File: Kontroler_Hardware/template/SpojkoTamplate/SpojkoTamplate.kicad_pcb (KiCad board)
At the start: 2 copper layers, 139.7 x 63.5 mm, 1 part, among them J1 CONN_01X40

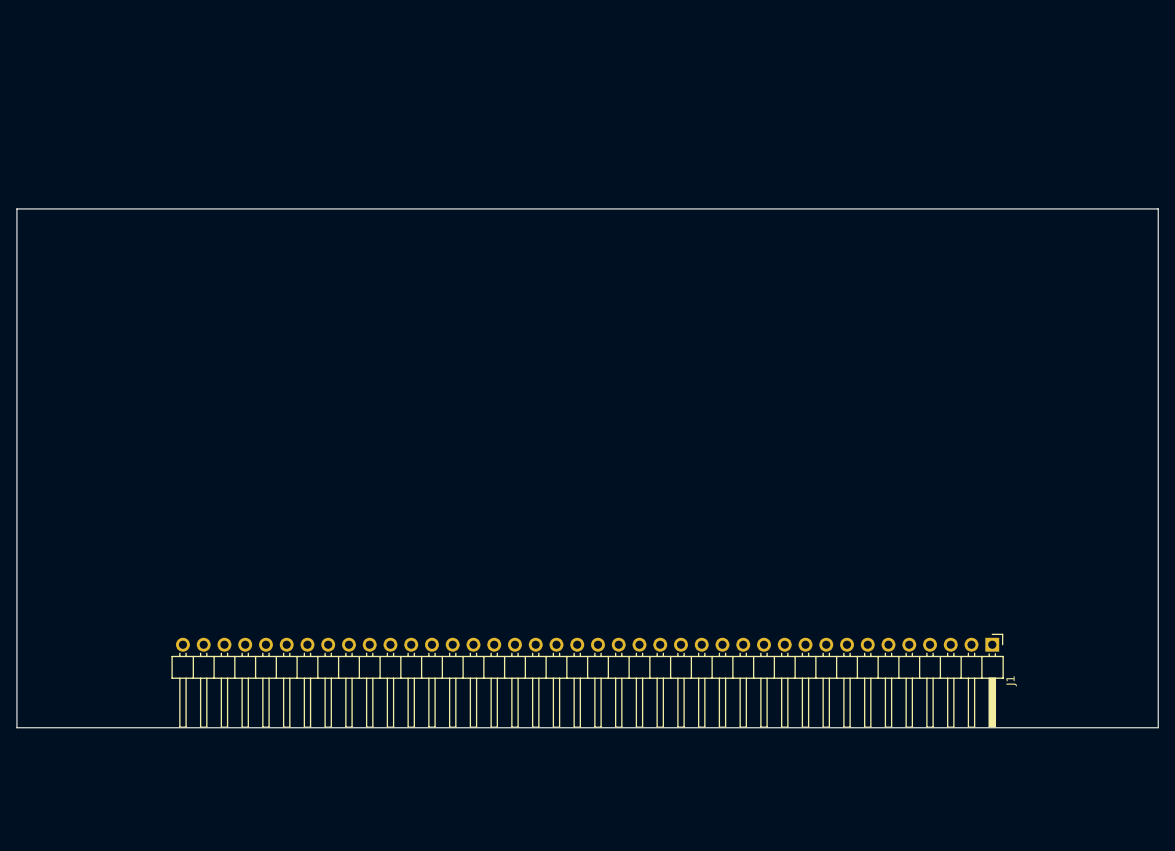
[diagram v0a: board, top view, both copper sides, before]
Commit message: Finish templates
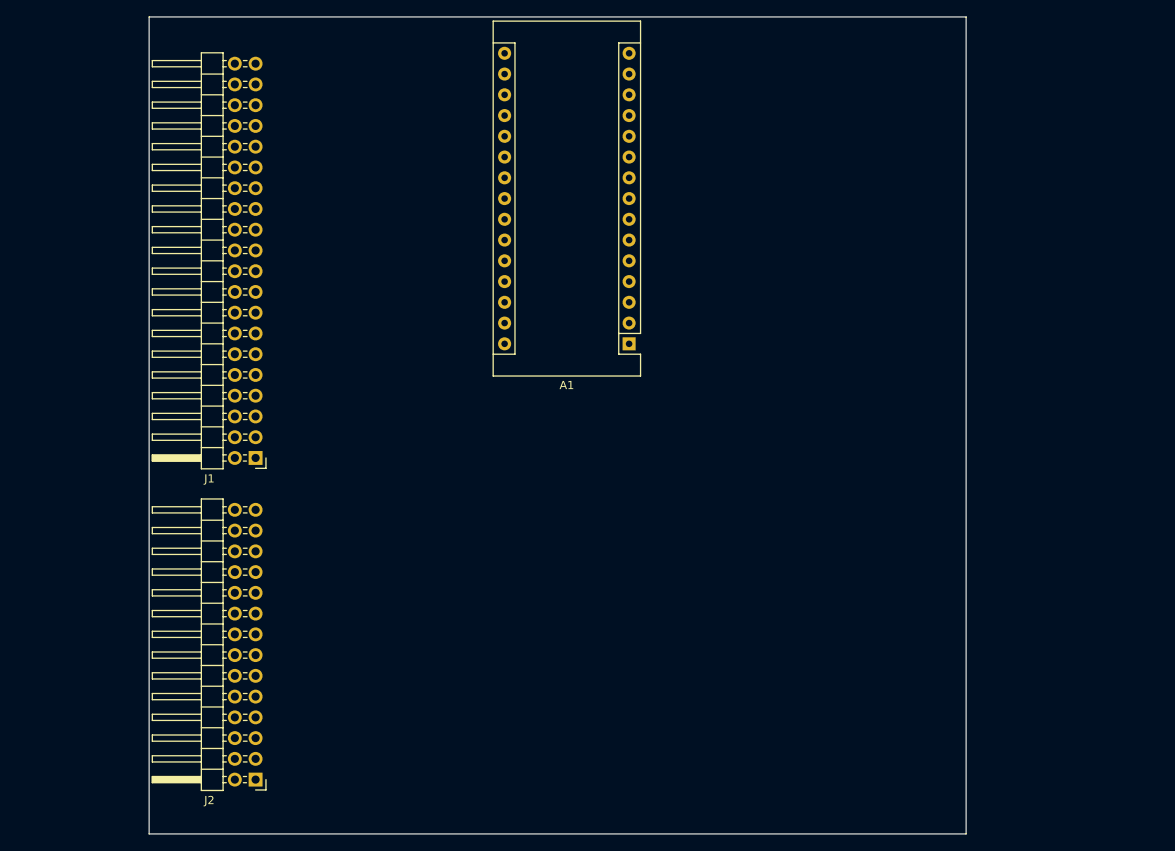
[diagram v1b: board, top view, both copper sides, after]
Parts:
- added A1: Arduino_Nano_v3.x, Module:Arduino_Nano, F.Cu at (158.8, 80.0)
- added J2: Conn_02x14_Odd_Even, Connector_PinHeader_2.54mm:PinHeader_2x14_P2.54mm_Horizontal, F.Cu at (113.0, 133.3)
- J1: value CONN_01X40 -> Conn_02x20_Odd_Even; footprint Pin_Headers:Pin_Header_Angled_1x40_Pitch2.54mm -> Connector_PinHeader_2.54mm:PinHeader_2x20_P2.54mm_Horizontal
- moved J1 93.0 mm to (113.0, 94.0), turned to 180 degrees
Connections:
- J1 pad 1: +24V -> GPIO21
- J1 pad 10: +3V3 -> GPIO25
- J1 pad 11: +3V3 -> GPIO24
- J1 pad 12: GND -> GPIO24
- J1 pad 13: GND -> GPIO23
- J1 pad 14: GPIO21 -> GPIO23
- J1 pad 15: GPIO20 -> GPIO18
- J1 pad 16: GPIO16 -> GPIO18
- J1 pad 17: GPIO12 -> GND
- J1 pad 18: GPIO25 -> GND
- J1 pad 19: GPIO24 -> RST
- J1 pad 2: +24V -> GPIO21
- J1 pad 20: GPIO23 -> RST
- J1 pad 21: GPIO18 -> GND
- J1 pad 22: Net-(J1-Pad22) -> GND
- J1 pad 23: Net-(J1-Pad23) -> TXD
- J1 pad 24: Net-(J1-Pad24) -> TXD
- J1 pad 25: Net-(J1-Pad25) -> RXD
- J1 pad 26: Net-(J1-Pad26) -> RXD
- J1 pad 27: Net-(J1-Pad27) -> GND
- J1 pad 28: Net-(J1-Pad28) -> GND
- J1 pad 29: Net-(J1-Pad29) -> SDA1
- J1 pad 3: +24V -> GPIO20
- J1 pad 30: GND -> SDA1
- J1 pad 31: RST -> SCL1
- J1 pad 32: GND -> SCL1
- J1 pad 33: TXD -> GND
- J1 pad 34: RXD -> GND
- J1 pad 35: GND -> SDA
- J1 pad 36: SCL1 -> SDA
- J1 pad 37: SDA1 -> SCL
- J1 pad 38: GND -> SCL
- J1 pad 39: SDA -> GND
- J1 pad 4: +24V -> GPIO20
- J1 pad 40: SCL -> GND
- J1 pad 5: GND -> GPIO16
- J1 pad 6: GND -> GPIO16
- J1 pad 7: +5V -> GPIO12
- J1 pad 8: +5V -> GPIO12
- J1 pad 9: GND -> GPIO25
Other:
- board size 139.7 x 63.5 mm -> 100 x 100 mm
